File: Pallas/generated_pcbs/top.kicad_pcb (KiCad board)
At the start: 2 copper layers, 467.5 x 140 mm, 19 parts

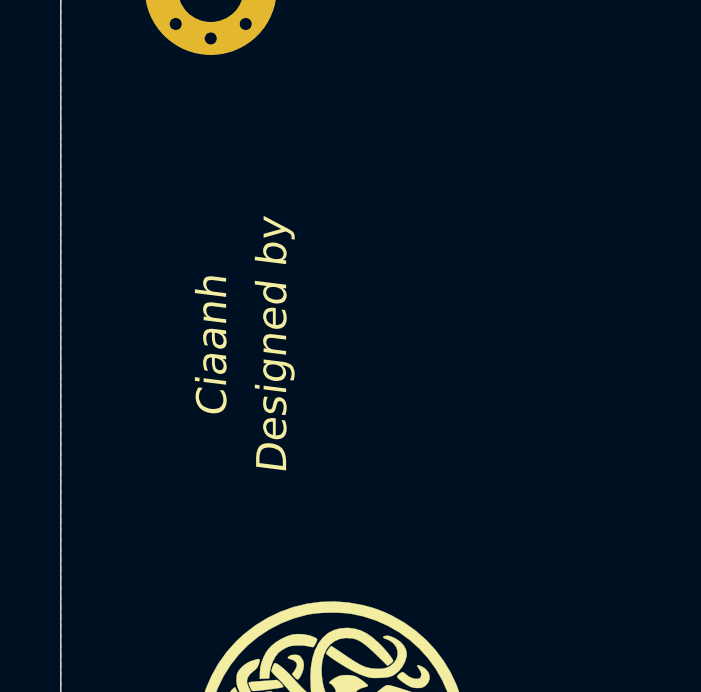
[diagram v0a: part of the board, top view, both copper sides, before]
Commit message: Fix issue with label design by
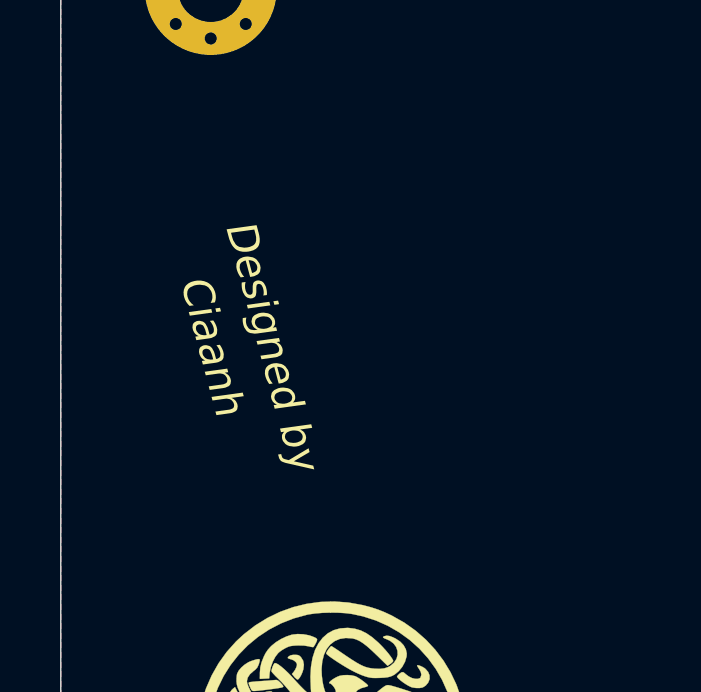
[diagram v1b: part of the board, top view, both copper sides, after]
